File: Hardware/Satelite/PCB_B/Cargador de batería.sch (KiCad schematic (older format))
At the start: 6 parts, among them U10 BQ21040DBVR

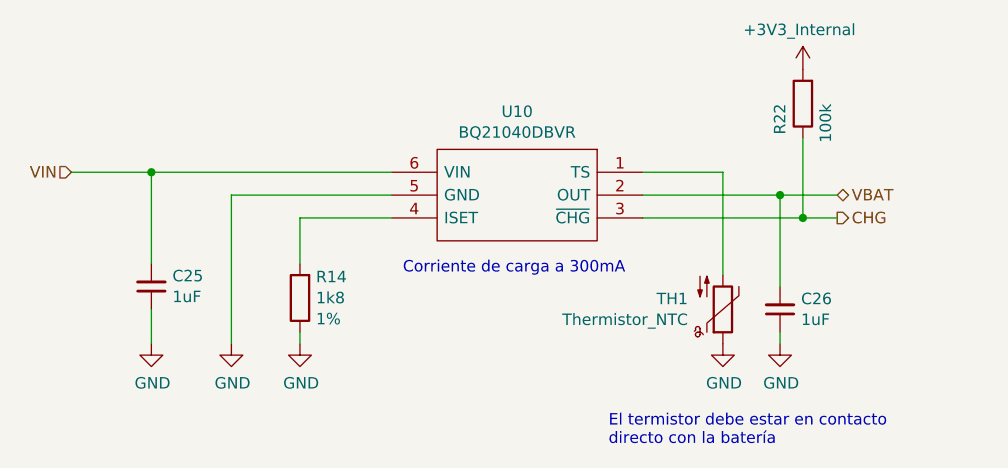
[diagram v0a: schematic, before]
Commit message: PCB_B V2 terminado
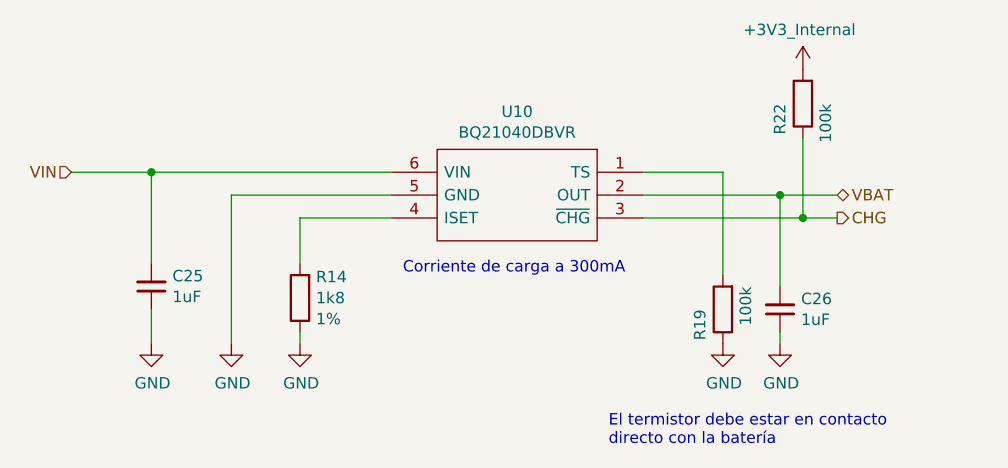
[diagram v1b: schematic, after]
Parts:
- removed TH1: Thermistor_NTC, Resistor_SMD:R_0603_1608Metric_Pad1.05x0.95mm_HandSolder, symbol Device:Thermistor_NTC
- added R19: 100k, Resistor_SMD:R_0603_1608Metric_Pad1.05x0.95mm_HandSolder, symbol Device:R
- U10: footprint SOT95P280X145-6N -> SamacSys_Parts:SOT95P280X145-6N
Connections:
- net GND: now also R19.1
- net at U10.1 (TS): now also R19.2
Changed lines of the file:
@@
 F 0 "U10" H 6900 3815 50  0000 C CNN
 F 1 "BQ21040DBVR" H 6900 3724 50  0000 C CNN
-F 2 "SOT95P280X145-6N" H 7300 3650 50  0001 L CNN
+F 2 "SamacSys_Parts:SOT95P280X145-6N" H 7300 3650 50  0001 L CNN
 F 3 "http://www.ti.com/lit/gpn/bq21040" H 7300 3550 50  0001 L CNN
 F 4 "0.8A Single Input Single-Cell Li-Ion and Li-Pol Battery Charger" H 7300 3450 50  0001 L CNN "Description"
@@
 	7050 3750 6350 3750
 $Comp
-L Device:Thermistor_NTC TH1
-U 1 1 5CC9077E
-P 6700 4150
-F 0 "TH1" H 6547 4104 50  0000 R CNN
-F 1 "Thermistor_NTC" H 6547 4195 50  0000 R CNN
-F 2 "Resistor_SMD:R_0603_1608Metric_Pad1.05x0.95mm_HandSolder" H 6700 4200 50  0001 C CNN
-F 3 "~" H 6700 4200 50  0001 C CNN
-F 4 "P12013CT-ND" H 6700 4150 50  0001 C CNN "Manufacturer Part Number"
-	1    6700 4150
-	1    0    0    1
-$EndComp
-$Comp
 L power:GND #PWR?
 U 1 1 5CC95641
@@
 Text Notes 6200 4750 0    50   ~ 0
 El termistor debe estar en contacto\ndirecto con la batería
+$Comp
+L Device:R R?
+U 1 1 5CD36697
+P 6700 4150
+AR Path="/5BA17F9C/5CD36697" Ref="R?"  Part="1"
+AR Path="/5BA1A7F9/5CD36697" Ref="R?"  Part="1"
+AR Path="/5BA1A77A/5CD36697" Ref="R?"  Part="1"
+AR Path="/5BC300BF/5CD36697" Ref="R19"  Part="1"
+F 0 "R19" V 6800 4150 50  0000 L CNN
+F 1 "100k" V 6600 4050 50  0000 L CNN
+F 2 "Resistor_SMD:R_0603_1608Metric_Pad1.05x0.95mm_HandSolder" V 6630 4150 50  0001 C CNN
+F 3 "~" H 6700 4150 50  0001 C CNN
+F 4 "RC0603JR-07100KL" V 6700 4150 50  0001 C CNN "Manufacturer Part Number"
+	1    6700 4150
+	-1   0    0    1
+$EndComp
 $EndSCHEMATC
